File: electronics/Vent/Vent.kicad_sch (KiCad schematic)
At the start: 1 part, among them U1 ESP32-C3-WROOM-02-N4

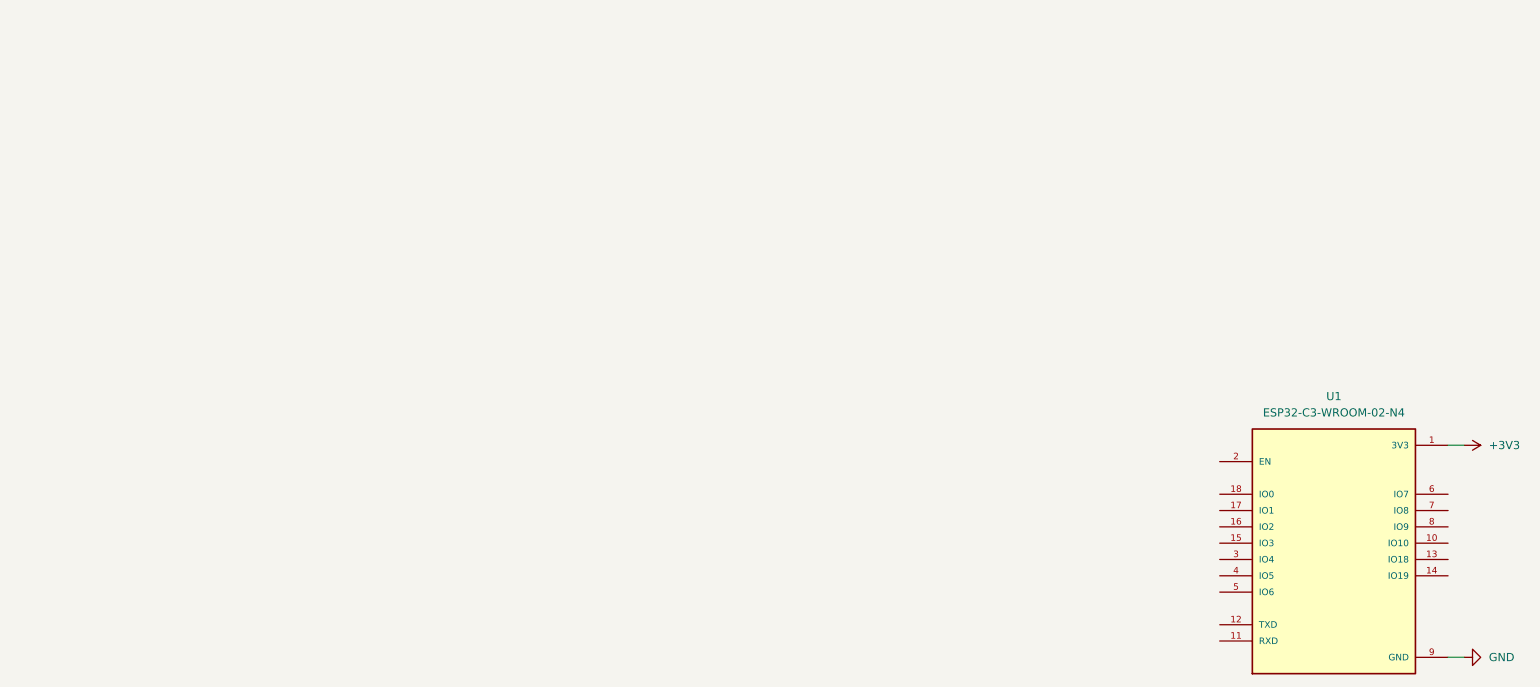
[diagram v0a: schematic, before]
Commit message: Autoprogramming, Finish off BMS, Add comps to Vent, and do a bunch of mobile stuff
Original-author: Zachariah K. Sharma <zachariah.sharma@gmail.com>
Source-commit: c8fb455aabb0719517b46fd9304eb5e5fb9f4004
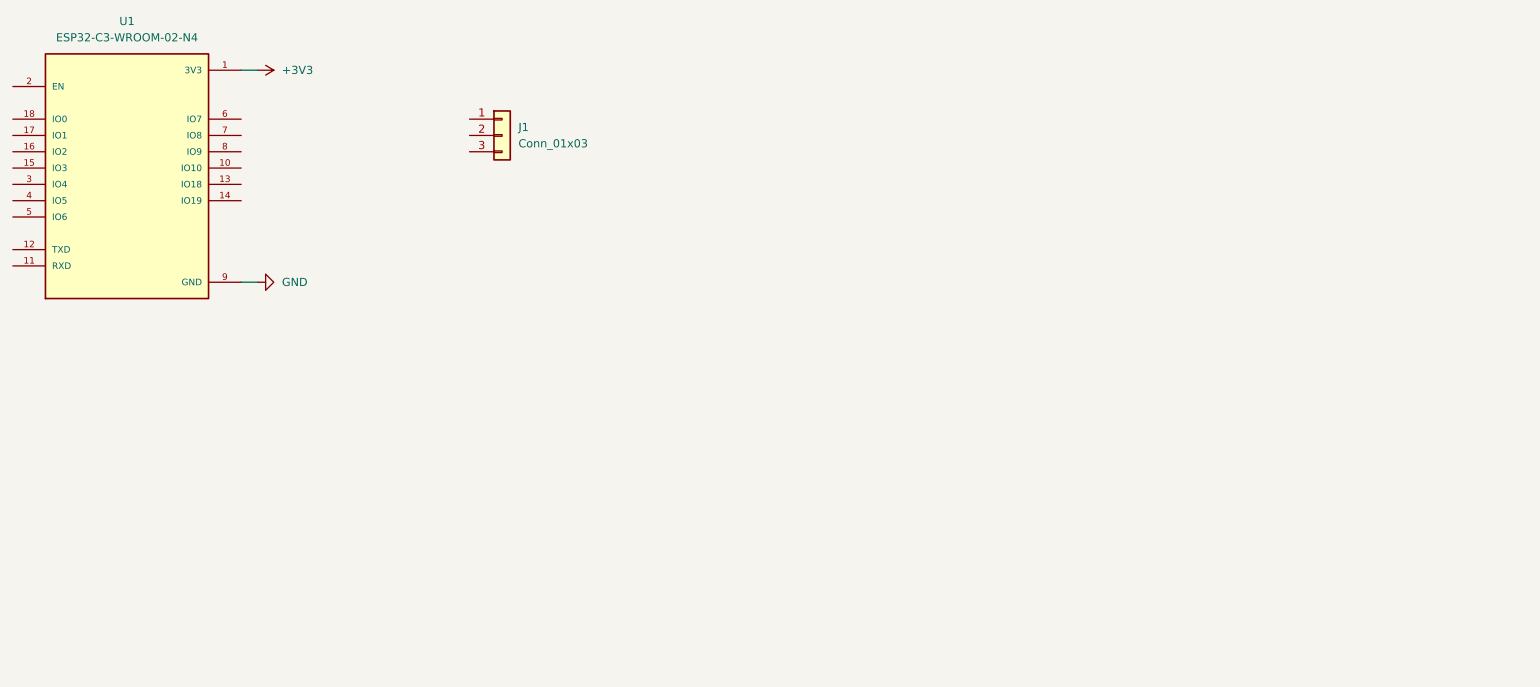
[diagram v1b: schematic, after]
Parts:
- added J1: Conn_01x03, Connector_PinHeader_1.00mm:PinHeader_1x03_P1.00mm_Vertical, symbol Connector_Generic:Conn_01x03
- U1: footprint ESP32-C3-WROOM-02-N4:MODULE_ESP32-C3-WROOM-02-H4 -> Footprints:MODULE_ESP32-C3-WROOM-02-H4
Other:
- moved on the sheet: U1
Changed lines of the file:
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@@
 	(wire
 		(pts
-			(xy 260.35 91.44) (xy 262.89 91.44)
+			(xy 72.39 33.02) (xy 74.93 33.02)
 		)
 		(stroke
@@
 	(wire
 		(pts
-			(xy 260.35 124.46) (xy 262.89 124.46)
+			(xy 72.39 66.04) (xy 74.93 66.04)
 		)
 		(stroke
@@
 	(symbol
 		(lib_id "power:+3V3")
-		(at 262.89 91.44 270)
+		(at 74.93 33.02 270)
 		(unit 1)
 		(exclude_from_sim no)
@@
 		(fields_autoplaced yes)
 		(property "Reference" "#PWR01"
-			(at 259.08 91.44 0)
+			(at 71.12 33.02 0)
 			(effects
 				(font
@@
 		)
 		(property "Value" "+3V3"
-			(at 266.7 91.4399 90)
+			(at 78.74 33.0199 90)
 			(effects
 				(font
@@
 		)
 		(property "Footprint" ""
-			(at 262.89 91.44 0)
+			(at 74.93 33.02 0)
 			(effects
 				(font
@@
 		)
 		(property "Datasheet" ""
-			(at 262.89 91.44 0)
+			(at 74.93 33.02 0)
 			(effects
 				(font
@@
 		)
 		(property "Description" "Power symbol creates a global label with name \"+3V3\""
-			(at 262.89 91.44 0)
+			(at 74.93 33.02 0)
 			(effects
 				(font
@@
 	(symbol
 		(lib_id "power:GND")
-		(at 262.89 124.46 90)
+		(at 74.93 66.04 90)
 		(unit 1)
 		(exclude_from_sim no)
@@
 		(fields_autoplaced yes)
 		(property "Reference" "#PWR02"
-			(at 269.24 124.46 0)
+			(at 81.28 66.04 0)
 			(effects
 				(font
@@
 		)
 		(property "Value" "GND"
-			(at 266.7 124.4599 90)
+			(at 78.74 66.0399 90)
 			(effects
 				(font
@@
 		)
 		(property "Footprint" ""
-			(at 262.89 124.46 0)
+			(at 74.93 66.04 0)
 			(effects
 				(font
@@
 		)
 		(property "Datasheet" ""
-			(at 262.89 124.46 0)
+			(at 74.93 66.04 0)
 			(effects
 				(font
@@
 		)
 		(property "Description" "Power symbol creates a global label with name \"GND\" , ground"
-			(at 262.89 124.46 0)
+			(at 74.93 66.04 0)
 			(effects
 				(font
@@
 	(symbol
 		(lib_id "ESP32-C3-WROOM-02-N4:ESP32-C3-WROOM-02-N4")
-		(at 242.57 109.22 0)
+		(at 54.61 50.8 0)
 		(unit 1)
 		(exclude_from_sim no)
@@
 		(fields_autoplaced yes)
 		(property "Reference" "U1"
-			(at 242.57 83.82 0)
+			(at 54.61 25.4 0)
 			(effects
 				(font
@@
 		)
 		(property "Value" "ESP32-C3-WROOM-02-N4"
-			(at 242.57 86.36 0)
-			(effects
-				(font
-					(size 1.27 1.27)
-				)
-			)
-		)
-		(property "Footprint" "ESP32-C3-WROOM-02-N4:MODULE_ESP32-C3-WROOM-02-H4"
-			(at 242.57 109.22 0)
+			(at 54.61 27.94 0)
+			(effects
+				(font
+					(size 1.27 1.27)
+				)
+			)
+		)
+		(property "Footprint" "Footprints:MODULE_ESP32-C3-WROOM-02-H4"
+			(at 54.61 50.8 0)
 			(effects
 				(font
@@
 		)
 		(property "Datasheet" ""
-			(at 242.57 109.22 0)
+			(at 54.61 50.8 0)
 			(effects
 				(font
@@
 		)
 		(property "Description" ""
-			(at 242.57 109.22 0)
+			(at 54.61 50.8 0)
 			(effects
 				(font
@@
 		)
 		(property "MF" "Espressif Systems"
-			(at 242.57 109.22 0)
+			(at 54.61 50.8 0)
 			(effects
 				(font
@@
 		)
 		(property "DESCRIPTION" "WiFi Modules (802.11) (Engineering Samples) SMD module, ESP32-C3, 4MB SPI flash, PCB antenna, -40 C +105 C"
-			(at 242.57 109.22 0)
+			(at 54.61 50.8 0)
 			(effects
 				(font
@@
 		)
 		(property "PACKAGE" "Package"
-			(at 242.57 109.22 0)
+			(at 54.61 50.8 0)
 			(effects
 				(font
@@
 		)
 		(property "PRICE" "None"
-			(at 242.57 109.22 0)
+			(at 54.61 50.8 0)
 			(effects
 				(font
@@
 		)
 		(property "Package" "Package"
-			(at 242.57 109.22 0)
+			(at 54.61 50.8 0)
 			(effects
 				(font
@@
 		)
 		(property "Check_prices" "https://www.snapeda.com/parts/ESP32-C3-WROOM-02-N4/Espressif+Systems/view-part/?ref=eda"
-			(at 242.57 109.22 0)
+			(at 54.61 50.8 0)
 			(effects
 				(font
@@
 		)
 		(property "Price" "None"
-			(at 242.57 109.22 0)
+			(at 54.61 50.8 0)
 			(effects
 				(font
@@
 		)
 		(property "SnapEDA_Link" "https://www.snapeda.com/parts/ESP32-C3-WROOM-02-N4/Espressif+Systems/view-part/?ref=snap"
-			(at 242.57 109.22 0)
+			(at 54.61 50.8 0)
 			(effects
 				(font
@@
 		)
 		(property "MP" "ESP32-C3-WROOM-02-N4"
-			(at 242.57 109.22 0)
+			(at 54.61 50.8 0)
 			(effects
 				(font
@@
 		)
 		(property "Description_1" "WiFi Modules (802.11) (Engineering Samples) SMD module, ESP32-C3, 4MB SPI flash, PCB antenna, -40 C +85 C"
-			(at 242.57 109.22 0)
+			(at 54.61 50.8 0)
 			(effects
 				(font
@@
 		)
 		(property "Availability" "In Stock"
-			(at 242.57 109.22 0)
+			(at 54.61 50.8 0)
 			(effects
 				(font
@@
 		)
 		(property "AVAILABILITY" "In Stock"
-			(at 242.57 109.22 0)
+			(at 54.61 50.8 0)
 			(effects
 				(font
@@
 		)
 		(property "PURCHASE-URL" "https://pricing.snapeda.com/search/part/ESP32-C3-WROOM-02-H4/?ref=eda"
-			(at 242.57 109.22 0)
+			(at 54.61 50.8 0)
 			(effects
 				(font
@@
 					(unit 1)
 				)
+			)
+		)
+	)
+	(symbol
+		(lib_id "Connector_Generic:Conn_01x03")
+		(at 113.03 43.18 0)
+		(unit 1)
+		(exclude_from_sim no)
+		(in_bom yes)
+		(on_board yes)
+		(dnp no)
+		(fields_autoplaced yes)
+		(property "Reference" "J1"
+			(at 115.57 41.9099 0)
+			(effects
+				(font
+					(size 1.27 1.27)
+				)
+				(justify left)
+			)
+		)
+		(property "Value" "Conn_01x03"
+			(at 115.57 44.4499 0)
+			(effects
+				(font
+					(size 1.27 1.27)
+				)
+				(justify left)
+			)
+		)
+		(property "Footprint" "Connector_PinHeader_1.00mm:PinHeader_1x03_P1.00mm_Vertical"
+			(at 113.03 43.18 0)
+			(effects
+				(font
+					(size 1.27 1.27)
+				)
+				(hide yes)
+			)
+		)
+		(property "Datasheet" "~"
+			(at 113.03 43.18 0)
+			(effects
+				(font
+					(size 1.27 1.27)
+				)
+				(hide yes)
+			)
+		)
+		(property "Description" "Generic connector, single row, 01x03, script generated (kicad-library-utils/schlib/autogen/connector/)"
+			(at 113.03 43.18 0)
+			(effects
+				(font
+					(size 1.27 1.27)
+				)
+				(hide yes)
+			)
+		)
+		(pin "2"
+		)
+		(pin "1"
+		)
+		(pin "3"
+		)
+		(instances
+			(project ""
+				(path "/ea2bda2b-bb9a-4e5a-ab88-7882822440d3"
+					(reference "J1")
+					(unit 1)
+				)
